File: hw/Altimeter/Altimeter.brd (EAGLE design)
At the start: 49.3 x 20.3 mm, 58 parts, among them U1 ATSAMD21G-A, U2 MPU-9250, U3 MS5803-14BA, X1 22-23-2041, X2 22-23-2041, Y1 32.768kHx

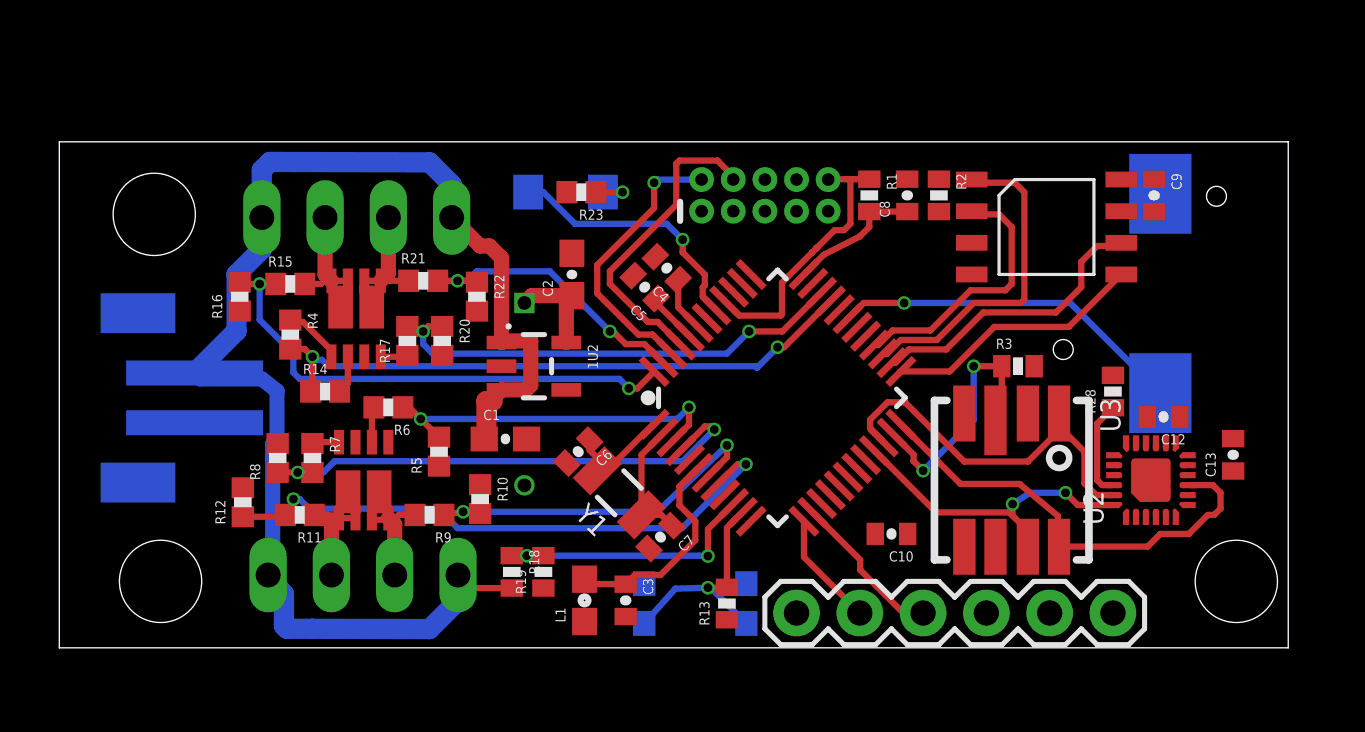
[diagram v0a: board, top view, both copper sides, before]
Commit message: dasAltimeter
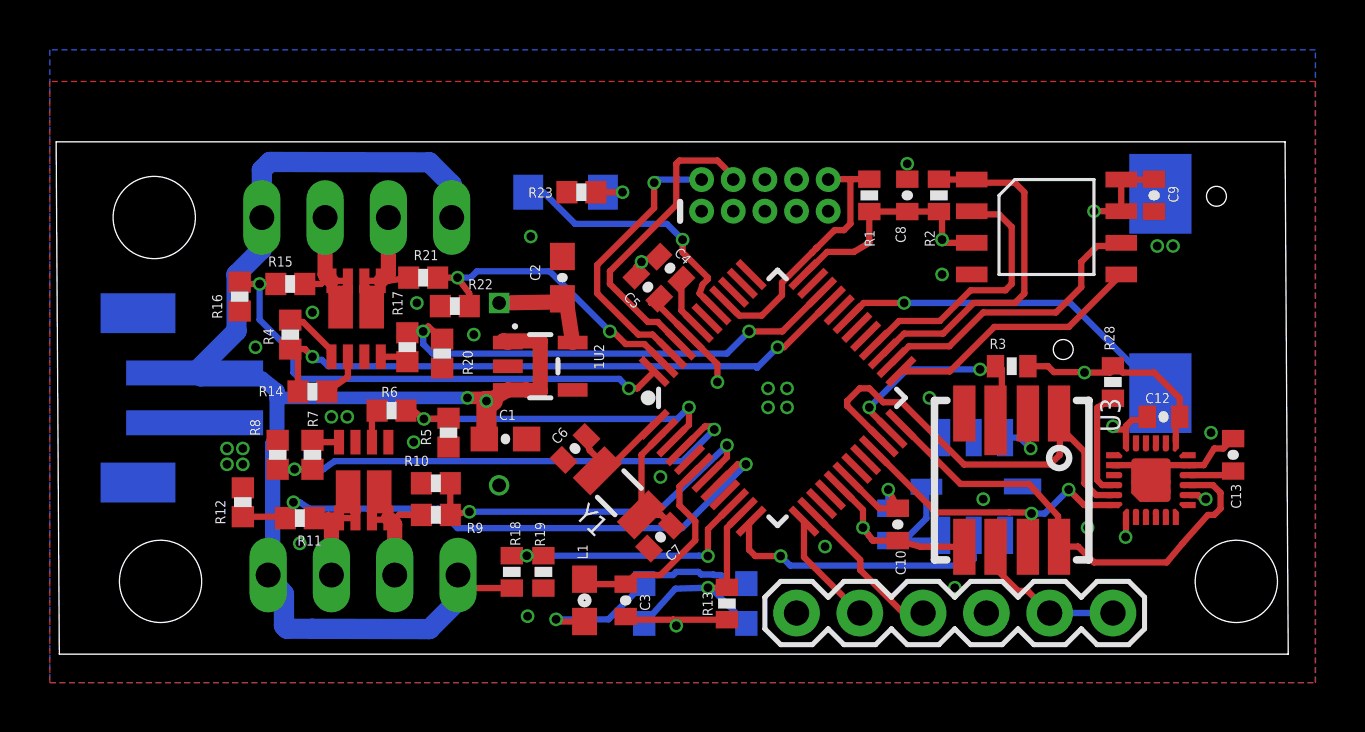
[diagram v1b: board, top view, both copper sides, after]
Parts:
- added C16: 0.1uF, SparkFun-Passives:0402-CAP
- added U$7: ADXL193, SparkFun-Sensors:ADXL193
- moved R10 1.89 mm to (18.0, 9.27), turned to 0 degrees
- moved U$1 1.02 mm to (20.6, 16.5)
- moved R22 0.97 mm to (18.8, 16.4), turned to 180 degrees
- moved R5 0.85 mm to (18.5, 11.3)
- moved R14 0.51 mm to (13.1, 13.0)
- moved R20 0.51 mm to (18.3, 14.5)
- moved C10 0.46 mm to (36.6, 7.62), turned to 90 degrees
- moved C2 0.40 mm to (23.1, 17.5)
- moved R28 0.38 mm to (45.2, 13.3)
- moved 1U2 0.25 mm to (22.2, 14.0)
- moved R17 0.25 mm to (16.9, 14.7)
- moved R3 0.25 mm to (41.1, 14.0)
- moved R9 0.25 mm to (18.0, 8.00)
- moved R6 0.18 mm to (16.3, 12.2)
- moved C6 0.18 mm to (23.6, 10.7)
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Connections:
- new net ACCELX: U$7.P$6, U1.12
- net 3.3V: now also C16.1, U$7.P$7, U$7.P$8
- net GND: now also C16.2, U$7.P$3
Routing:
- net 3.3V: track 11.8 -> 64.7 mm, vias 0 -> 8
- net GND: track 2.41 -> 28.7 mm, vias 0 -> 34
- net ACCELX: track 0.00 -> 11.5 mm, vias 0 -> 1
- net RAW: track 55.7 -> 59.1 mm, vias 0 -> 2
- net SPI1_SCK: track 15.2 -> 18.1 mm
- net REGOUT: track 0.00 -> 1.82 mm
- net CS_MEM: track 13.2 -> 14.4 mm
- net SPI1_MISO: track 18.1 -> 18.9 mm
- net CS_BARO: track 10.4 -> 9.75 mm
- net SPI1_MOSI: track 13.2 -> 12.7 mm
- net FET_C: track 4.14 -> 4.68 mm
- added copper zone on layer 15, net 3.3V
- added copper zone on layer 1, net GND
- added copper zone on layer 16, net GND
- added copper zone on layer 2, net GND
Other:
- board size 49.3 x 20.3 mm -> 49.5 x 20.6 mm
- board text added: "Altimeter?"

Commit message: working on sample libary and IMU
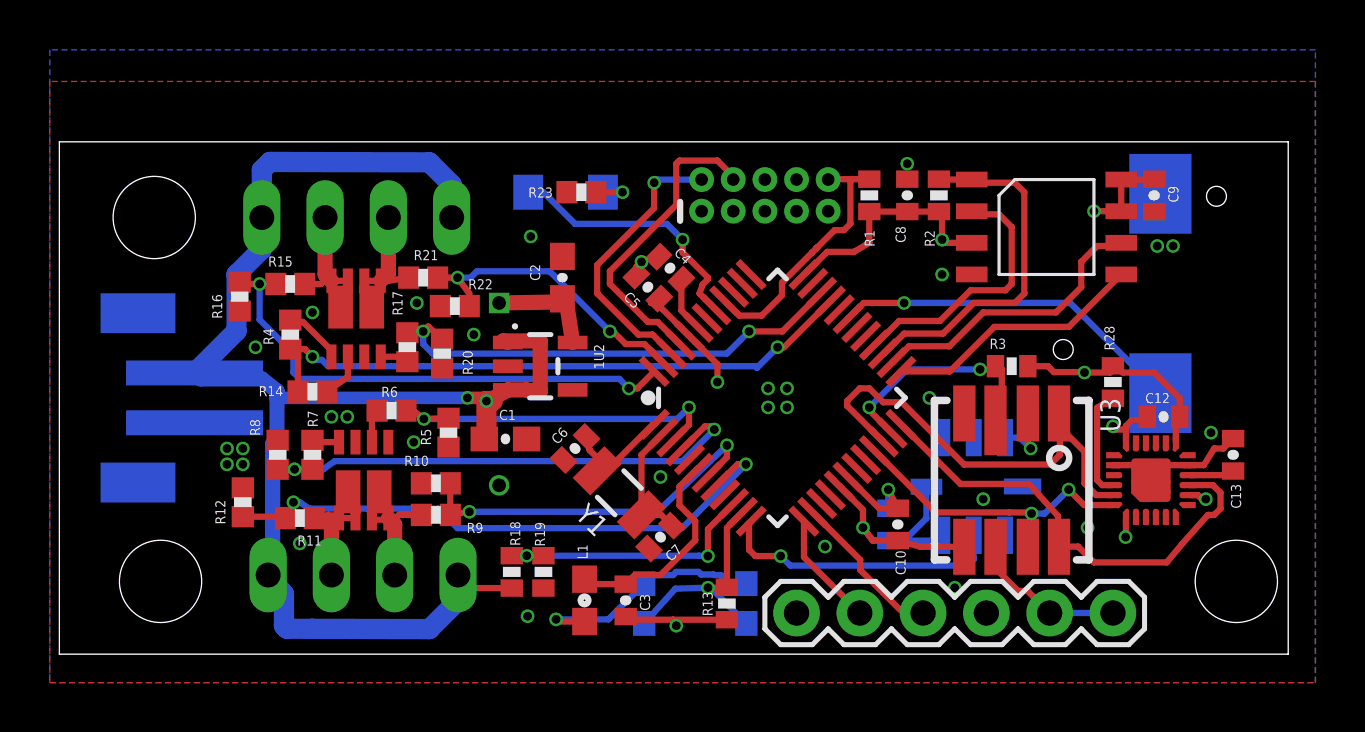
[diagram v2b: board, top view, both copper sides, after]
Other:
- board size 49.5 x 20.6 mm -> 49.3 x 20.6 mm
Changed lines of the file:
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@@
 <layer number="29" name="tStop" color="7" fill="3" visible="no" active="yes"/>
 <layer number="30" name="bStop" color="7" fill="6" visible="no" active="yes"/>
-<layer number="31" name="tCream" color="7" fill="4" visible="no" active="yes"/>
+<layer number="31" name="tCream" color="7" fill="4" visible="yes" active="yes"/>
 <layer number="32" name="bCream" color="7" fill="5" visible="no" active="yes"/>
 <layer number="33" name="tFinish" color="6" fill="3" visible="no" active="yes"/>
@@
 <plain>
 <wire x1="2.921" y1="2.413" x2="52.248" y2="2.413" width="0" layer="20"/>
-<wire x1="52.248" y1="2.413" x2="52.121" y2="22.977" width="0" layer="20"/>
-<wire x1="52.121" y1="22.977" x2="2.794" y2="22.977" width="0" layer="20"/>
-<wire x1="2.794" y1="22.977" x2="2.921" y2="2.413" width="0" layer="20"/>
+<wire x1="52.248" y1="2.413" x2="52.248" y2="22.977" width="0" layer="20"/>
+<wire x1="52.248" y1="22.977" x2="2.921" y2="22.977" width="0" layer="20"/>
+<wire x1="2.921" y1="22.977" x2="2.921" y2="2.413" width="0" layer="20"/>
 <text x="22.098" y="13.208" size="1.4224" layer="26" rot="MR0">Altimeter?</text>
 </plain>

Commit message: day one changes
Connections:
- net CS_IMU: now also U1.29
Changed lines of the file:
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@@
 <wire x1="44.577" y1="9.398" x2="44.577" y2="12.304" width="0.254" layer="1"/>
 <wire x1="44.577" y1="12.304" x2="45.212" y2="12.685" width="0.254" layer="1"/>
+<contactref element="U1" pad="29"/>
+<wire x1="35.28553125" y1="15.174871875" x2="44.577" y2="12.304" width="0" layer="19" extent="1-1"/>
 </signal>
 <signal name="CS_BARO">
